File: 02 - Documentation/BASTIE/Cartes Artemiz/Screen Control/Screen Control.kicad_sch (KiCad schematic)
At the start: 12 parts, among them J1 4P Droit 22-11-2042, J2 2P Droit 2-11-2022, J4 4P Droit 22-11-2042, J5 2P Droit 2-11-2022, J6 2P Droit 2-11-2022, J7 3P Droit 22-11-2032, U1 Teensy3.5

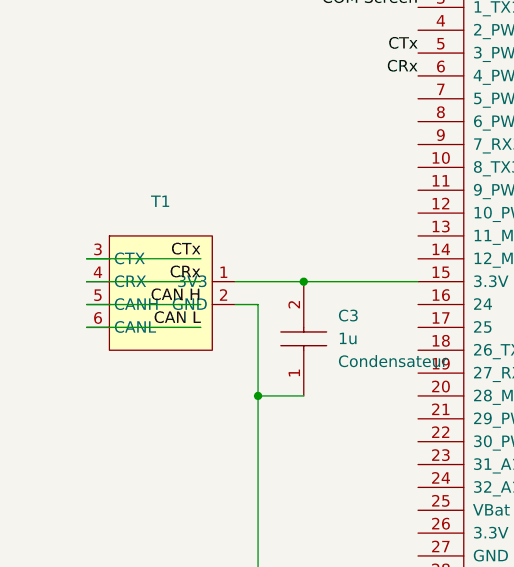
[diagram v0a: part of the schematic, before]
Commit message: Kicadlib + Modifs cartes
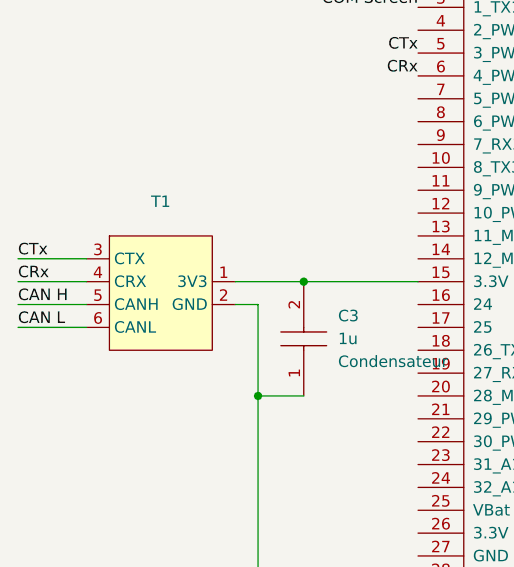
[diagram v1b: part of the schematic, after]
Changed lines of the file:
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@@
 	(wire
 		(pts
-			(xy 50.8 88.9) (xy 63.5 88.9)
+			(xy 50.8 88.9) (xy 43.18 88.9)
 		)
 		(stroke
@@
 	(wire
 		(pts
-			(xy 50.8 86.36) (xy 63.5 86.36)
+			(xy 50.8 86.36) (xy 43.18 86.36)
 		)
 		(stroke
@@
 	(wire
 		(pts
-			(xy 50.8 83.82) (xy 63.5 83.82)
+			(xy 50.8 83.82) (xy 43.18 83.82)
 		)
 		(stroke
@@
 	(wire
 		(pts
-			(xy 50.8 81.28) (xy 63.5 81.28)
+			(xy 50.8 81.28) (xy 43.18 81.28)
 		)
 		(stroke
@@
 	)
 	(label "CAN L"
-		(at 63.5 88.9 180)
-		(fields_autoplaced yes)
-		(effects
-			(font
-				(size 1.27 1.27)
-			)
-			(justify right bottom)
+		(at 43.18 88.9 0)
+		(fields_autoplaced yes)
+		(effects
+			(font
+				(size 1.27 1.27)
+			)
+			(justify left bottom)
 		)
 	)
@@
 	)
 	(label "CRx"
-		(at 63.5 83.82 180)
-		(fields_autoplaced yes)
-		(effects
-			(font
-				(size 1.27 1.27)
-			)
-			(justify right bottom)
+		(at 43.18 83.82 0)
+		(fields_autoplaced yes)
+		(effects
+			(font
+				(size 1.27 1.27)
+			)
+			(justify left bottom)
 		)
 	)
@@
 	)
 	(label "CTx"
-		(at 63.5 81.28 180)
-		(fields_autoplaced yes)
-		(effects
-			(font
-				(size 1.27 1.27)
-			)
-			(justify right bottom)
+		(at 43.18 81.28 0)
+		(fields_autoplaced yes)
+		(effects
+			(font
+				(size 1.27 1.27)
+			)
+			(justify left bottom)
 		)
 	)
@@
 	)
 	(label "CAN H"
-		(at 63.5 86.36 180)
-		(fields_autoplaced yes)
-		(effects
-			(font
-				(size 1.27 1.27)
-			)
-			(justify right bottom)
-		)
-	)
+		(at 43.18 86.36 0)
+		(fields_autoplaced yes)
+		(effects
+			(font
+				(size 1.27 1.27)
+			)
+			(justify left bottom)
+		)
+	)
